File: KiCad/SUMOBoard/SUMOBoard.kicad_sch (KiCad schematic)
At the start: 8 parts, among them J1 Conn_01x03_Socket, J2 Conn_01x03_Socket, J3 Conn_01x03_Socket, J4 Conn_01x03_Socket, J5 Conn_01x20_Pin, U1 Pico

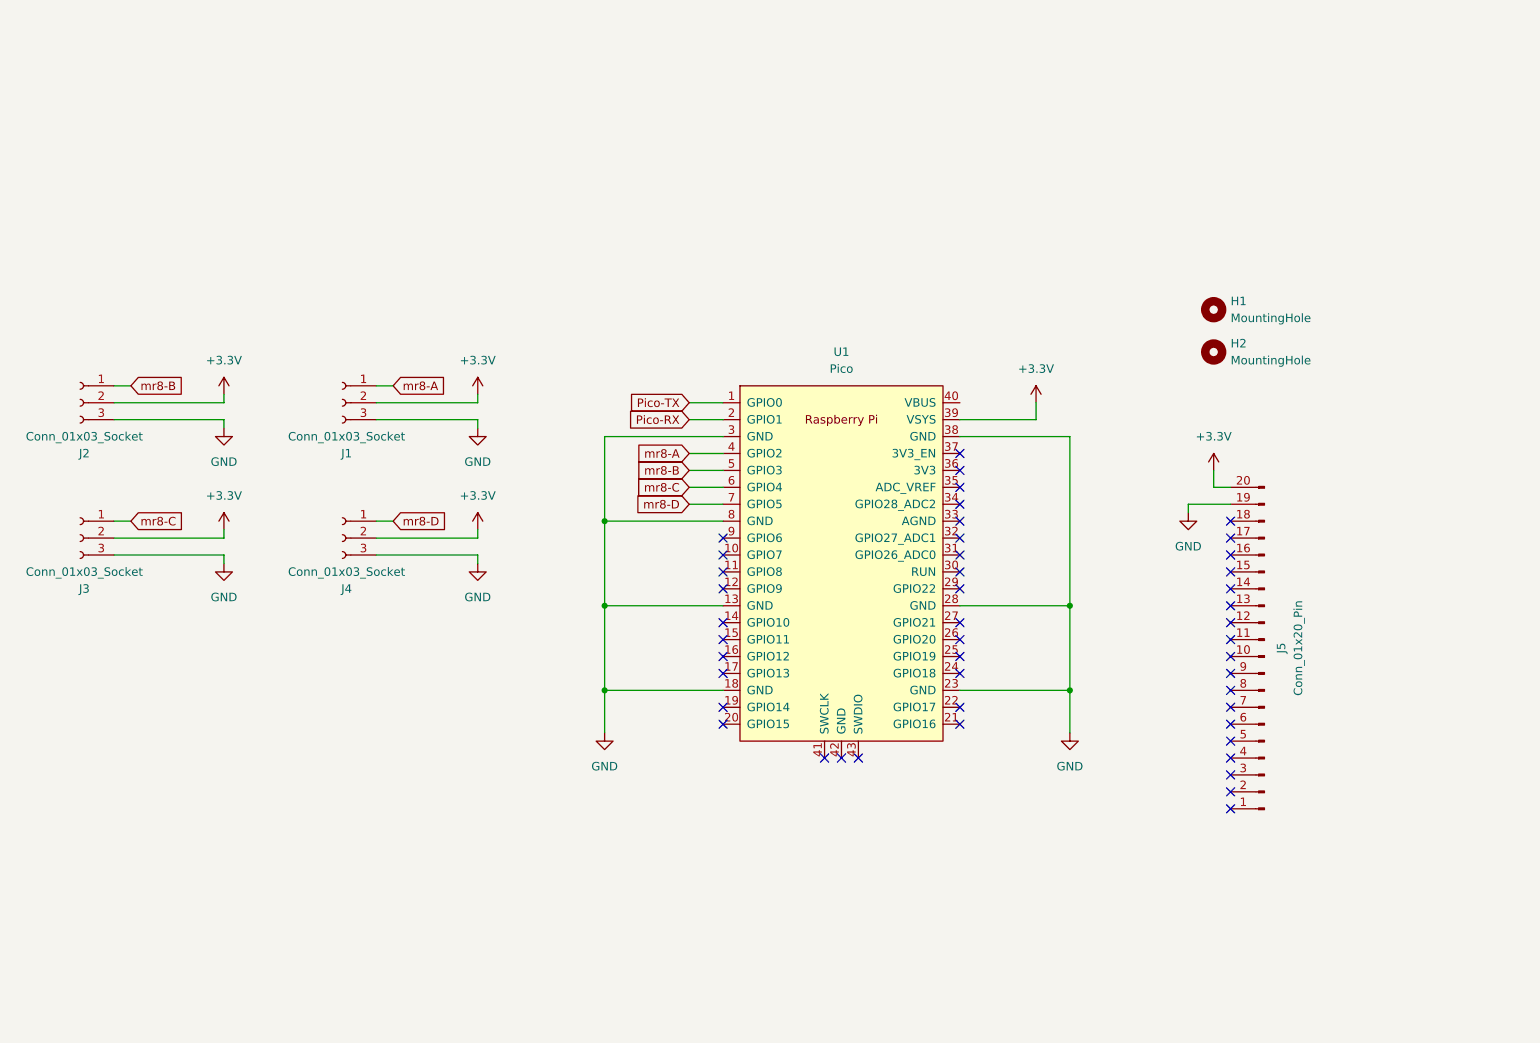
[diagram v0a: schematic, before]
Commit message: Build2作成
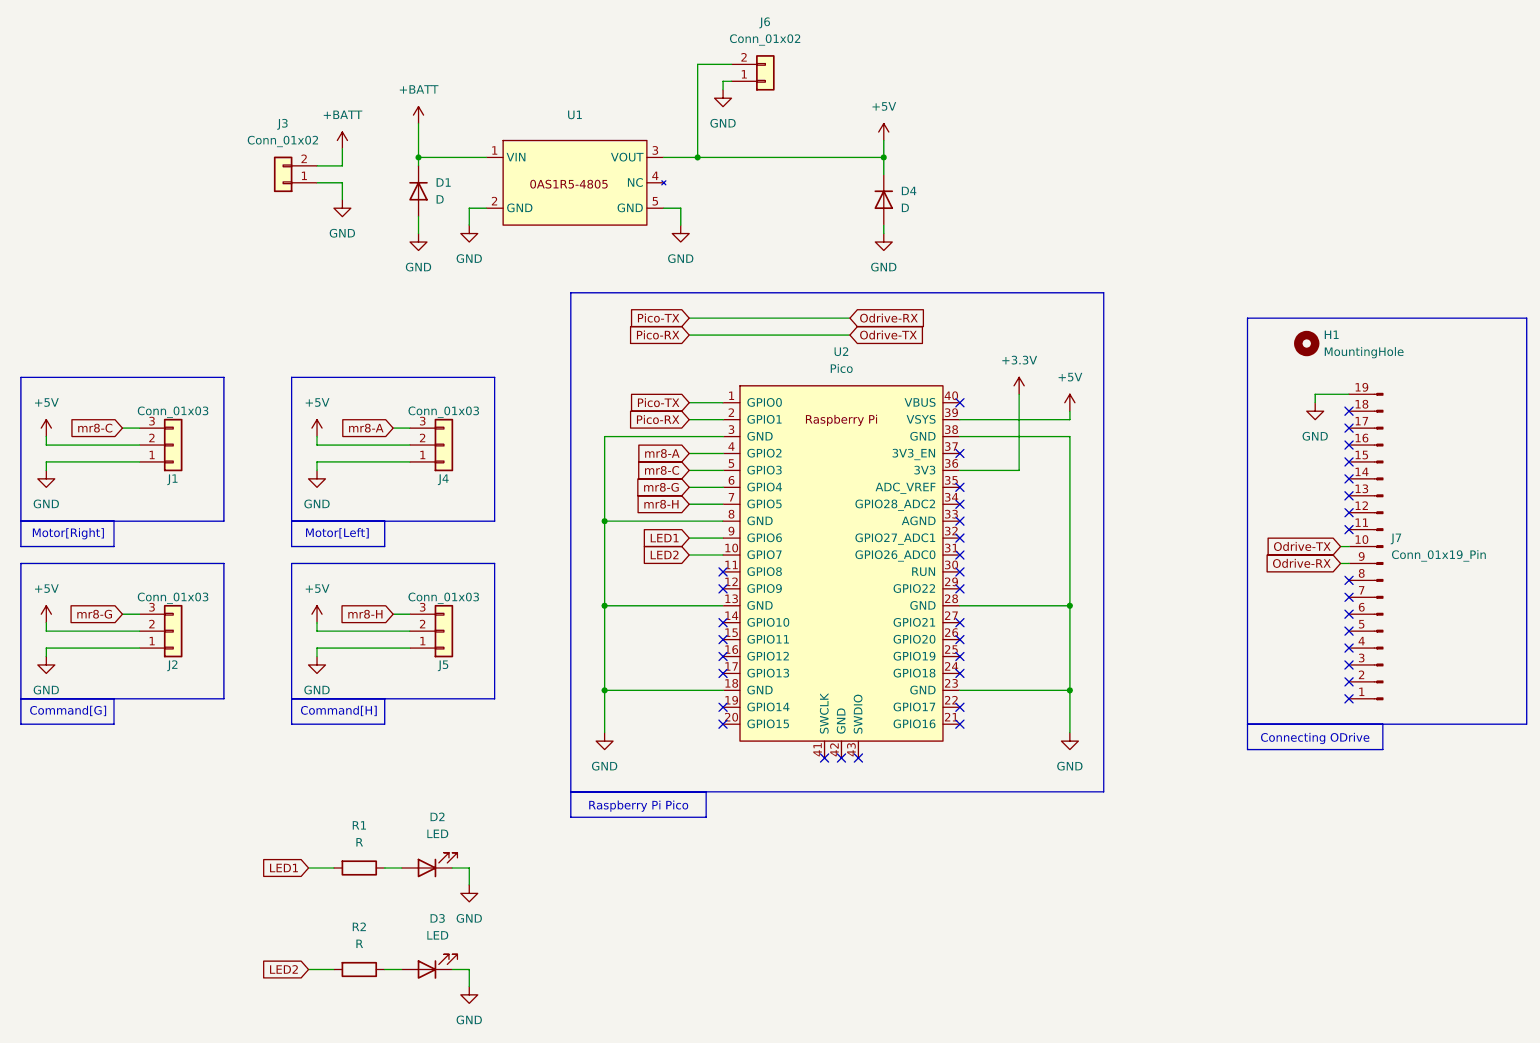
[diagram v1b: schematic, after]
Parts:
- removed H2: MountingHole, MountingHole:MountingHole_3.2mm_M3, symbol Mechanical:MountingHole
- removed J5: Conn_01x20_Pin, Connector_PinHeader_2.54mm:PinHeader_1x20_P2.54mm_Vertical, symbol Connector:Conn_01x20_Pin
- added D1, D4: D, Diode_SMD:D_SMA_Handsoldering, symbol Device:D
- added D2, D3: LED, LED_SMD:LED_0603_1608Metric_Pad1.05x0.95mm_HandSolder, symbol Device:LED
- added J3, J6: Conn_01x02, Connector_JST:JST_XH_B2B-XH-A_1x02_P2.50mm_Vertical, symbol Connector_Generic:Conn_01x02
- added J7: Conn_01x19_Pin, Connector_PinHeader_2.54mm:PinHeader_1x19_P2.54mm_Vertical, symbol Connector:Conn_01x19_Pin
- added R1, R2: R, Resistor_SMD:R_0603_1608Metric_Pad0.98x0.95mm_HandSolder, symbol Device:R
- added U1: ~, 0AS1R5-4805:0AS1R5-4805, symbol 0AS1R5-4805:0AS1R5-4805
- J1: renamed from J2; value Conn_01x03_Socket -> Conn_01x03; symbol Connector:Conn_01x03_Socket -> Connector_Generic:Conn_01x03
- J2: renamed from J3; value Conn_01x03_Socket -> Conn_01x03; footprint Connector_JST:JST_XH_B3B-XH-A_1x03_P2.50mm_Vertical -> (none); symbol Connector:Conn_01x03_Socket -> Connector_Generic:Conn_01x03
- J4: renamed from J1; value Conn_01x03_Socket -> Conn_01x03; symbol Connector:Conn_01x03_Socket -> Connector_Generic:Conn_01x03
- J5: renamed from J4; value Conn_01x03_Socket -> Conn_01x03; footprint Connector_JST:JST_XH_B3B-XH-A_1x03_P2.50mm_Vertical -> (none); symbol Connector:Conn_01x03_Socket -> Connector_Generic:Conn_01x03
- renumbered U1 to U2
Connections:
- net +3.3V: now also U2.36 (3V3); no longer J1.2 (Pin_2), J2.2 (Pin_2), J4.2 (Pin_2), J5.2 (Pin_2), U2.39 (VSYS)
- net GND: now also J1.1 (Pin_1), J2.1 (Pin_1), J4.1 (Pin_1), J5.1 (Pin_1), D1.2 (A), D2.1 (K), D3.1 (K), D4.2 (A), J3.1 (Pin_1), J6.1 (Pin_1), J7.19 (Pin_19), U1.2 (GND), U1.5 (GND); no longer J1.3 (Pin_3), J2.3 (Pin_3), J4.3 (Pin_3), J5.3 (Pin_3)
- net mr8-A: now also J4.3 (Pin_3); no longer J4.1 (Pin_1)
- net mr8-C: now also J1.3 (Pin_3), U2.5 (GPIO3); no longer J2.1 (Pin_1), U2.6 (GPIO4)
- net LED2: now reaches U2.10 (GPIO7)
- net LED2: now also R2.2
- net LED1: now reaches U2.9 (GPIO6)
- net LED1: now also R1.2
- net Pico-RX renamed Odrive-TX
- net Odrive-TX: now also J7.10 (Pin_10)
- net Pico-TX renamed Odrive-RX
- net Odrive-RX: now also J7.9 (Pin_9)
- removed net mr8-B: J1.1 (Pin_1), U2.5 (GPIO3)
- net mr8-D renamed mr8-H
- net mr8-H: now also J5.3 (Pin_3); no longer J5.1 (Pin_1)
- new net: D2.2 (A), R1.1
- new net: D3.2 (A), R2.1
- new net +5V: D4.1 (K), J1.2 (Pin_2), J2.2 (Pin_2), J4.2 (Pin_2), J5.2 (Pin_2), J6.2 (Pin_2), U1.3 (VOUT), U2.39 (VSYS)
- new net +BATT: D1.1 (K), J3.2 (Pin_2), U1.1 (VIN)
- new net mr8-G: J2.3 (Pin_3), U2.6 (GPIO4)
- no-connect marks 46 -> 42
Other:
- note added: "Command[G]"
- note added: "Command[H]"
- note added: "Connecting ODrive"
- note added: "Motor[Left]"
- note added: "Motor[Right]"
- note added: "Raspberry Pi Pico"
- moved on the sheet: H1
